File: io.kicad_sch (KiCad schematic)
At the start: 12 parts, among them J1 USB_C_Receptacle_USB2.0_16P, J3 Micro_SD_Card_Det_Hirose_DM3AT

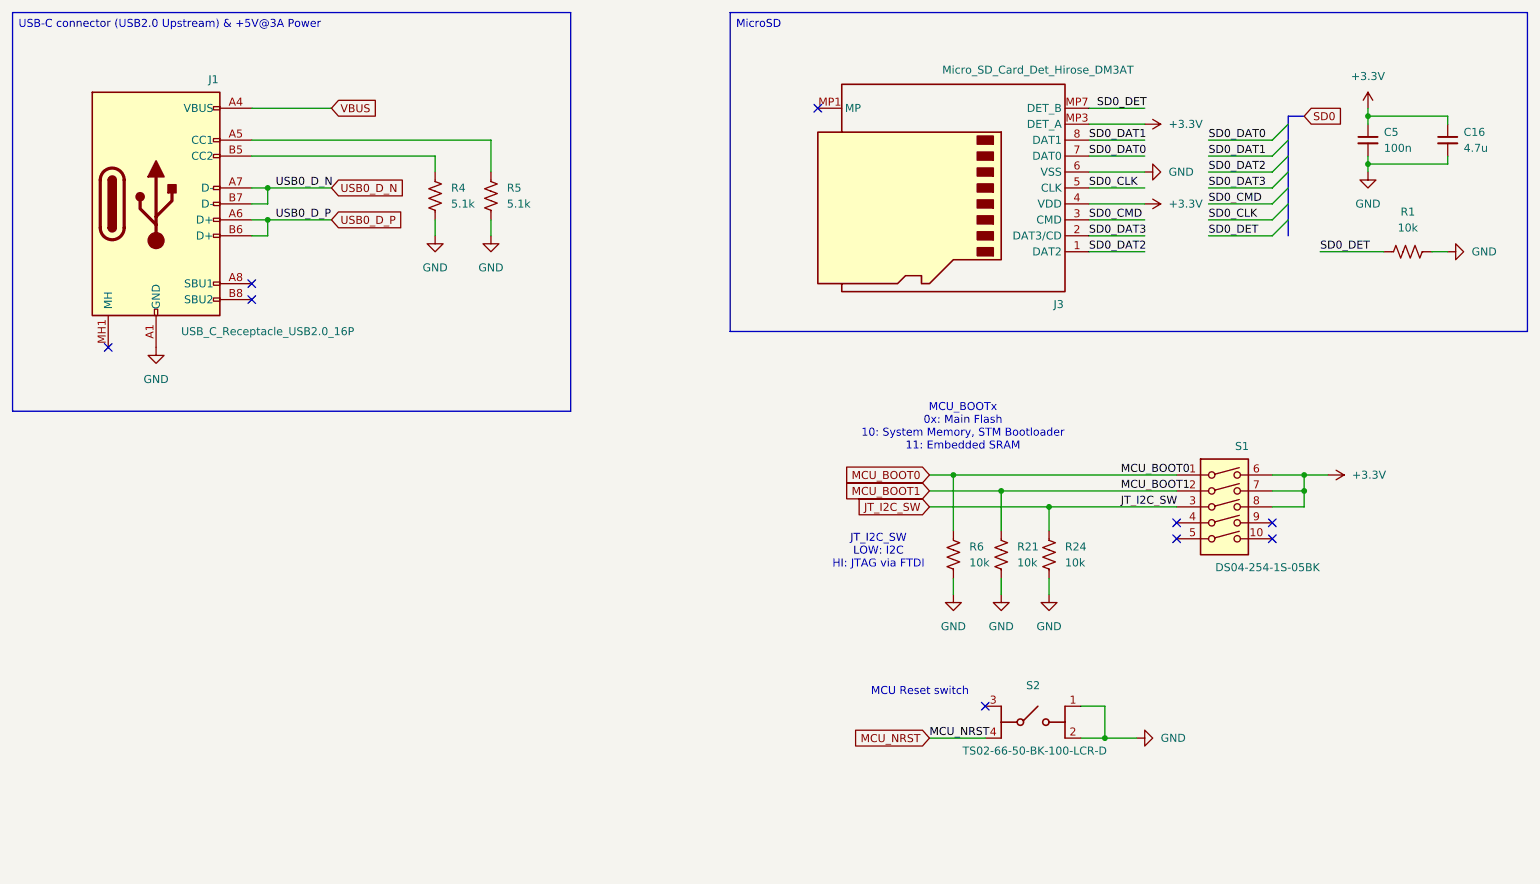
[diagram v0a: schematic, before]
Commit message: Stuff
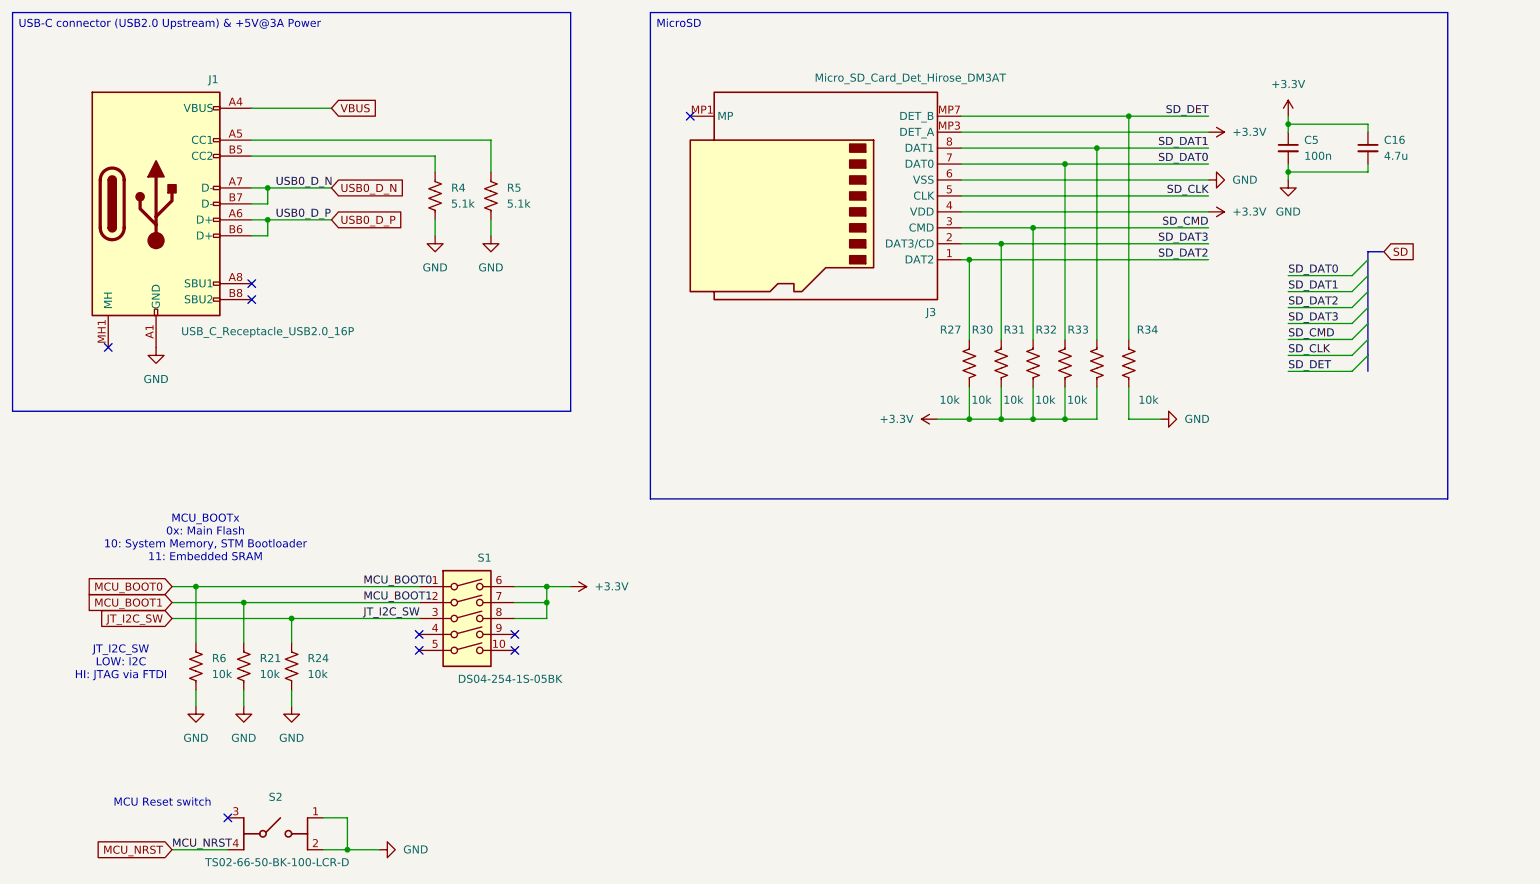
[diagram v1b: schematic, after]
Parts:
- removed R1: 10k, symbol Device:R_US
- added R27, R30, R31, R32, R33, R34: 10k, symbol Device:R_US
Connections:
- net +3.3V: now also R27.2, R30.2, R31.2, R32.2, R33.2
- net GND: now also R34.2
- net SD0_CLK renamed SD_CLK
- net SD0_CMD renamed SD_CMD
- net SD_CMD: now also R31.1
- net SD0_DAT0 renamed SD_DAT0
- net SD_DAT0: now also R32.1
- net SD0_DAT1 renamed SD_DAT1
- net SD_DAT1: now also R33.1
- net SD0_DAT2 renamed SD_DAT2
- net SD_DAT2: now also R27.1
- net SD0_DAT3 renamed SD_DAT3
- net SD_DAT3: now also R30.1
- net SD0_DET renamed SD_DET
- net SD_DET: now also R34.1
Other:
- moved on the sheet: C16, C5, J3, R21, R24, R6, S1, S2
